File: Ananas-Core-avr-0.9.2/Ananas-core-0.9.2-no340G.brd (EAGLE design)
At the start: 41.9 x 41.9 mm, 56 parts, among them U1 MYSMD_ATMEGA168-20AU, Y1-16/20MHZ MYSMD2_RESONATORMU

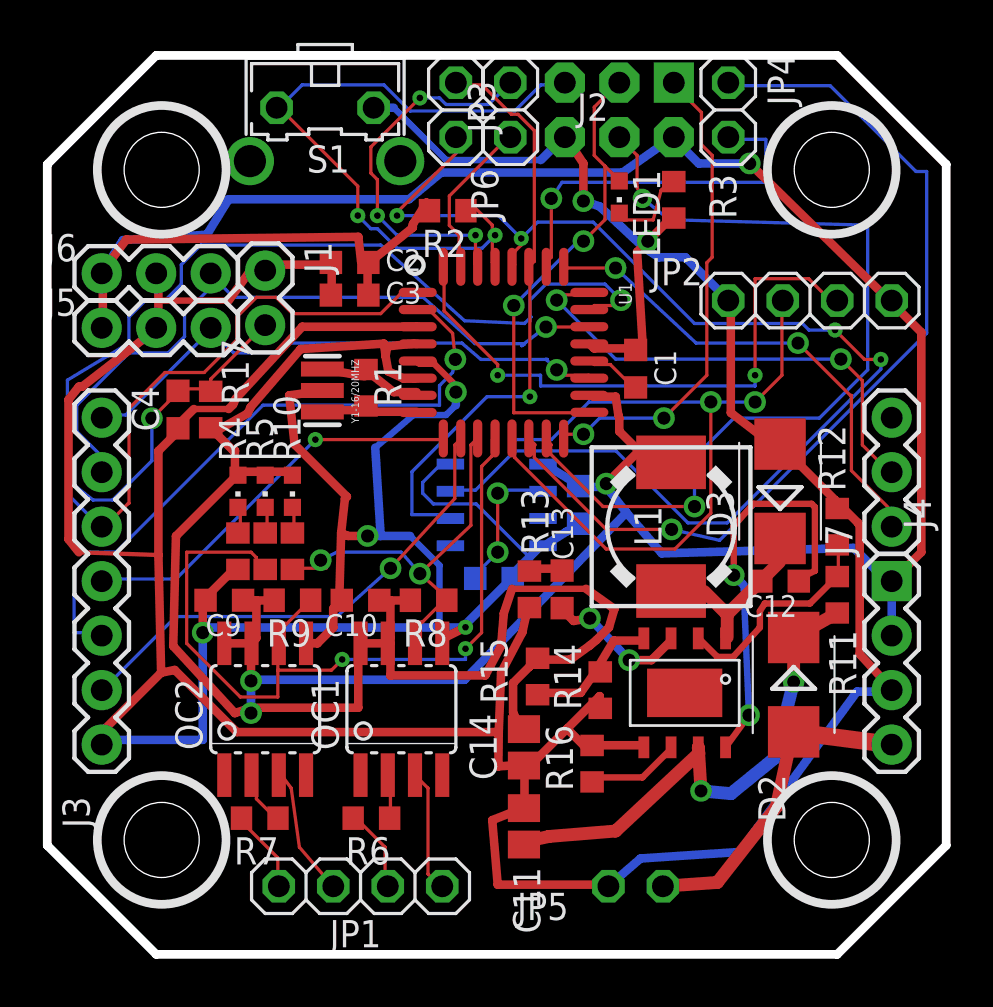
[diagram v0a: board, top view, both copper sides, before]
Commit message: fix the endstop
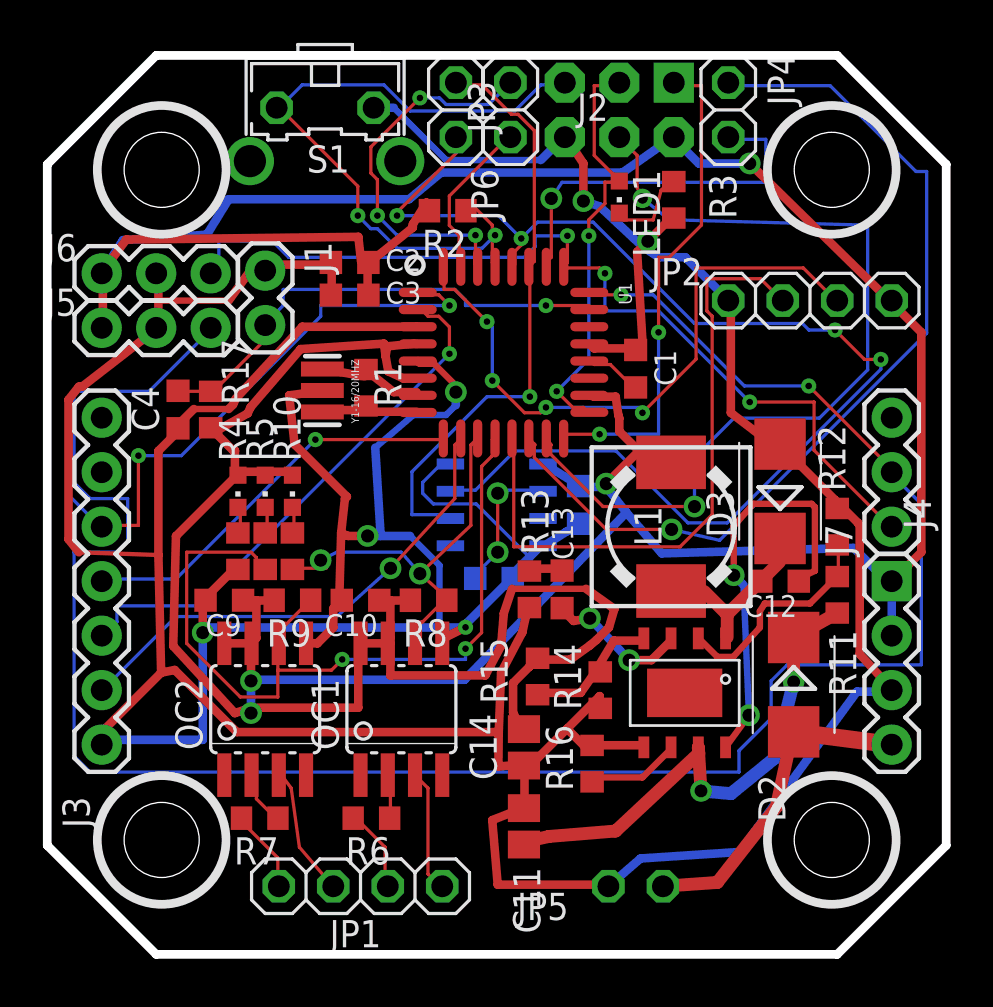
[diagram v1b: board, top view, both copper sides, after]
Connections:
- removed net S1: J3.7, J5.3, U1.19
- removed net S2: J3.6, J6.3, U1.22
- net DA: now also J6.3
- net DL: now also J5.3
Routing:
- net DL: track 22.6 -> 99.7 mm
- net S2: track 33.3 -> 0.00 mm, vias 1 -> 0
- net TEMP1: track 53.6 -> 22.7 mm, vias 2 -> 1
- net S1: track 26.2 -> 0.00 mm, vias 1 -> 0
- net DA: track 22.9 -> 43.1 mm, vias 2 -> 3
- net STEP_OUT: track 30.3 -> 25.1 mm
- net ENCODER_B: track 35.1 -> 30.0 mm, vias 2 -> 0
- net SCK: track 22.5 -> 19.5 mm
- net ENCODER_A: track 27.8 -> 29.5 mm, vias 2 -> 4
- net PWM: track 25.1 -> 26.4 mm, vias 0 -> 2
- net MISO: track 22.4 -> 23.3 mm
